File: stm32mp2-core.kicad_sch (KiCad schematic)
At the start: 0 parts

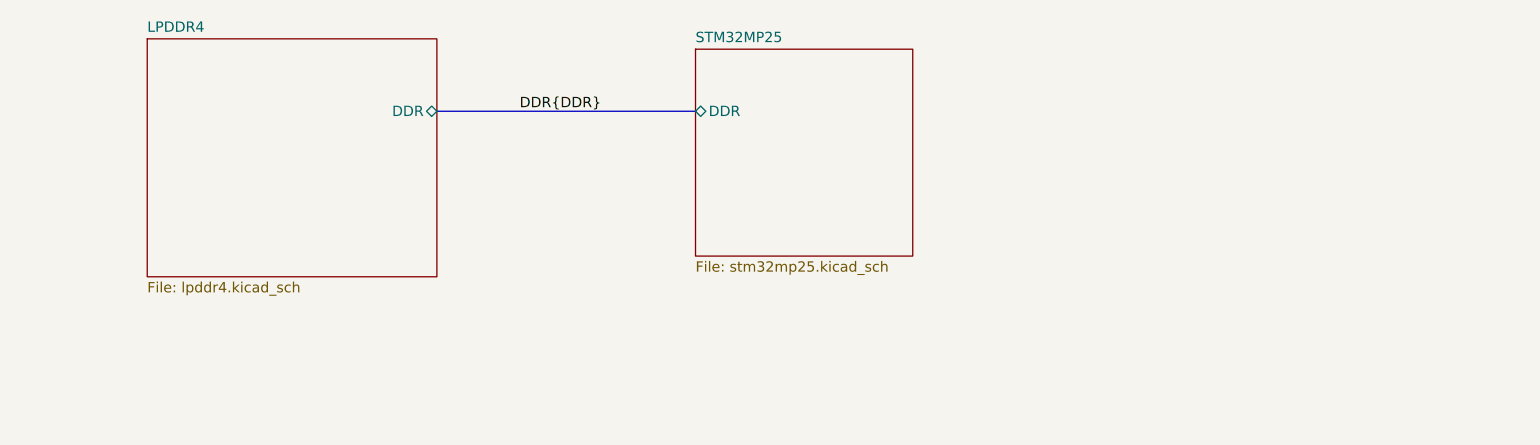
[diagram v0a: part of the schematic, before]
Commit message: got started on the pmic
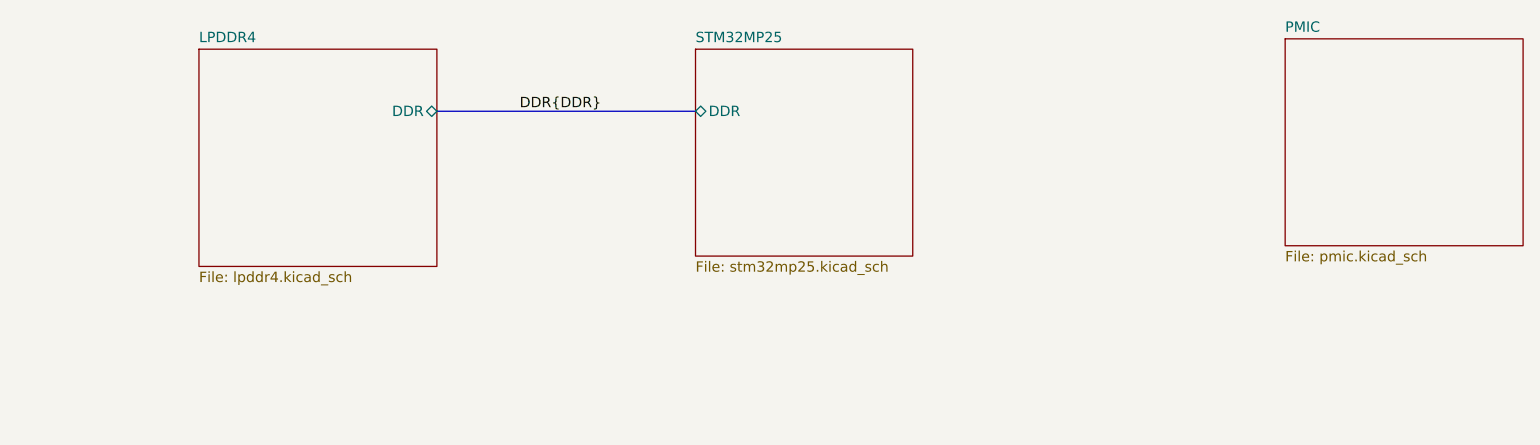
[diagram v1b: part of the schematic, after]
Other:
- added sheet PMIC (pmic.kicad_sch)
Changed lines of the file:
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@@
 	)
 	(sheet
-		(at 54.61 44.45)
-		(size 35.56 29.21)
+		(at 194.31 44.45)
+		(size 29.21 25.4)
+		(exclude_from_sim no)
+		(in_bom yes)
+		(on_board yes)
+		(dnp no)
+		(fields_autoplaced yes)
+		(stroke
+			(width 0.1524)
+			(type solid)
+		)
+		(fill
+			(color 0 0 0 0.0000)
+		)
+		(property "Sheetname" "PMIC"
+			(at 194.31 43.7384 0)
+			(effects
+				(font
+					(size 1.27 1.27)
+				)
+				(justify left bottom)
+			)
+		)
+		(property "Sheetfile" "pmic.kicad_sch"
+			(at 194.31 70.4346 0)
+			(effects
+				(font
+					(size 1.27 1.27)
+				)
+				(justify left top)
+			)
+		)
+		(instances
+			(project "stm32mp2-core"
+				(path "/5f8e630b-79db-437a-bc04-3ab5a18328d4"
+					(page "9")
+				)
+			)
+		)
+	)
+	(sheet
+		(at 60.96 45.72)
+		(size 29.21 26.67)
 		(exclude_from_sim no)
 		(in_bom yes)
@@
 		)
 		(property "Sheetname" "LPDDR4"
-			(at 54.61 43.7384 0)
+			(at 60.96 45.0084 0)
 			(effects
 				(font
@@
 		)
 		(property "Sheetfile" "lpddr4.kicad_sch"
-			(at 54.61 74.2446 0)
+			(at 60.96 72.9746 0)
 			(effects
 				(font
